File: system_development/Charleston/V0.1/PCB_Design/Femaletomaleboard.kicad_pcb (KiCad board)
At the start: 2 copper layers, 65 x 118.4 mm, 29 parts, among them SW2 MC74VHC1G66DFT1G

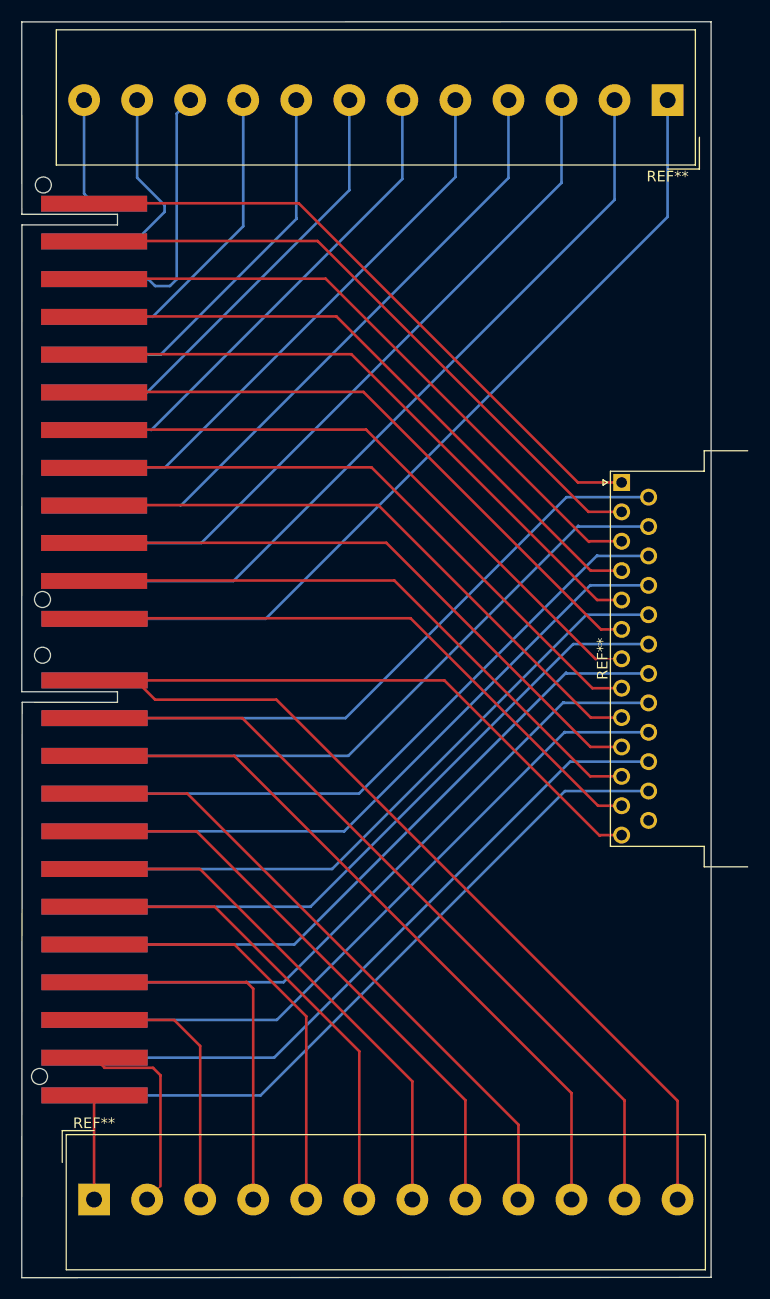
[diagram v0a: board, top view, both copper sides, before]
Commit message: Assembled Libraries
Assembled Libraries
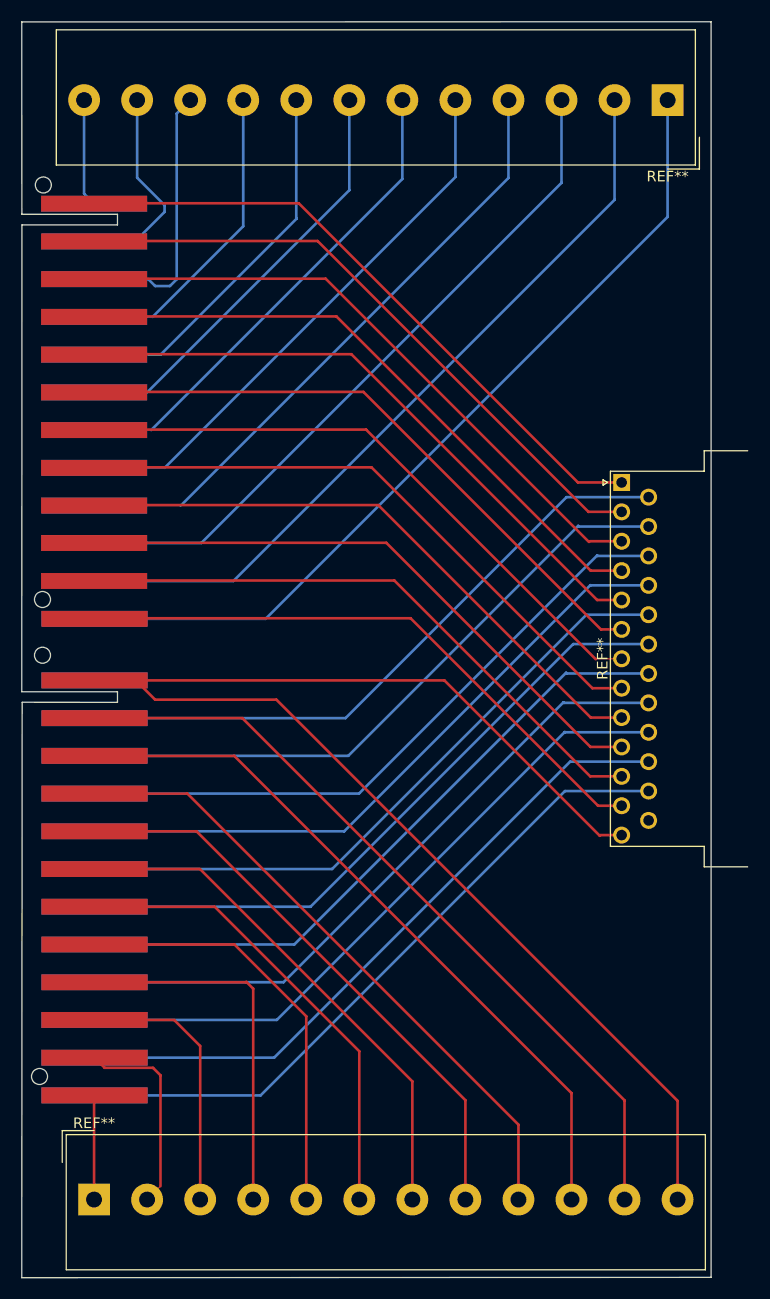
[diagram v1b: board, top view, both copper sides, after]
